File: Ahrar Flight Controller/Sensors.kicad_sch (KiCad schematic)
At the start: 38 parts, among them U3 MS5611-01BA, U5 BMP581

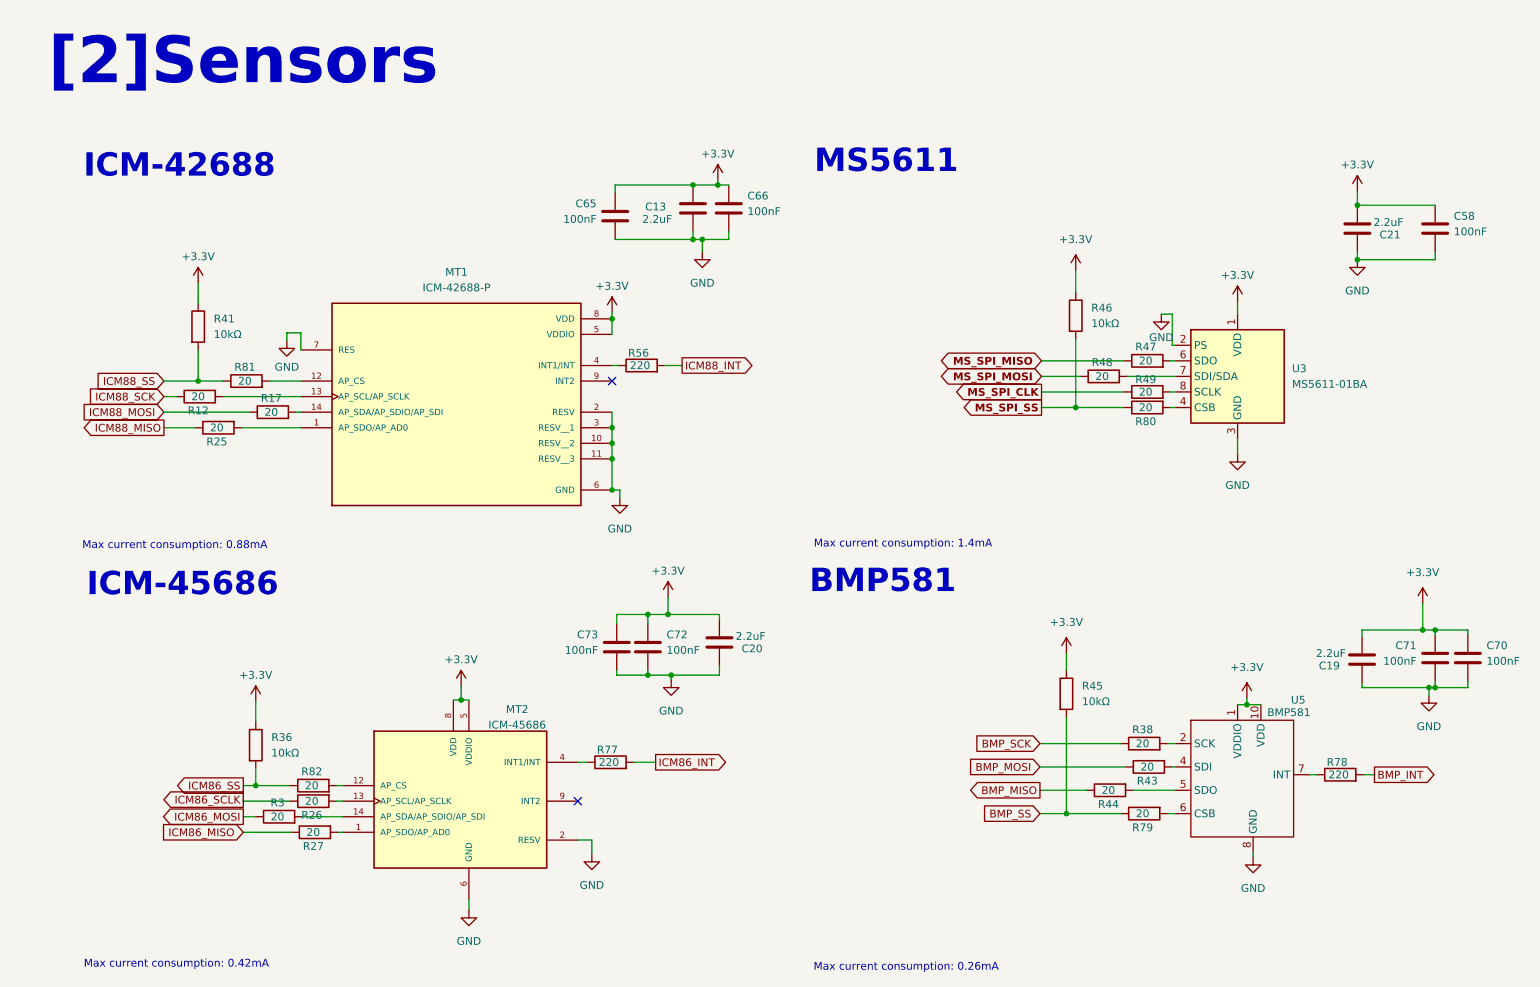
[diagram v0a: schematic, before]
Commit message: .
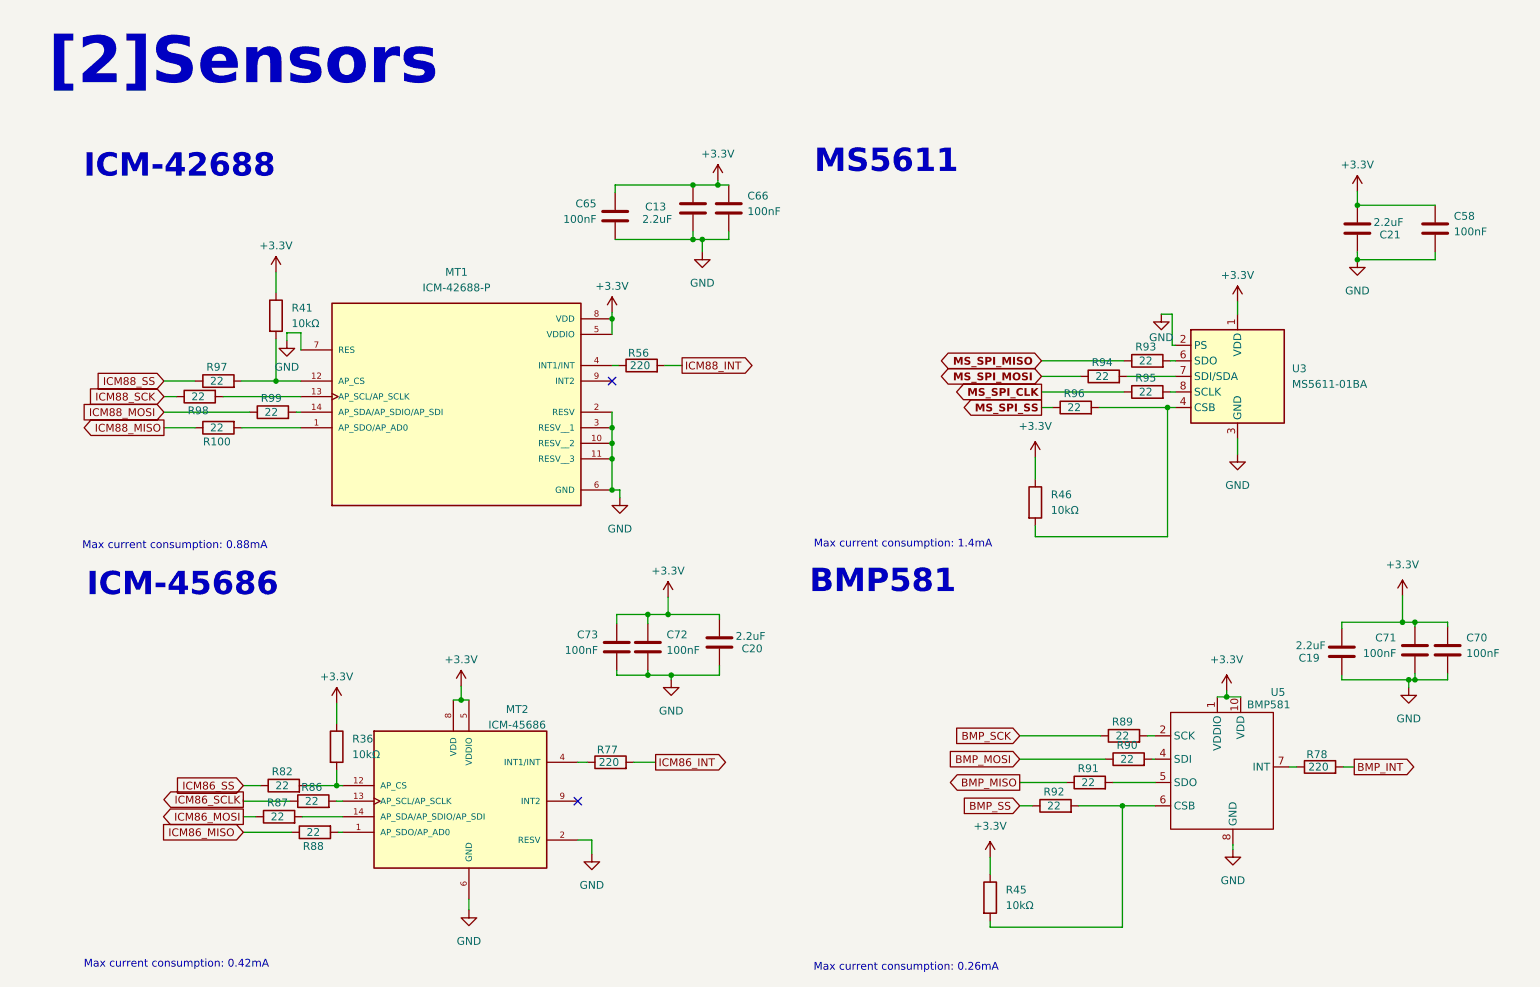
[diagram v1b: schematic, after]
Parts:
- removed R12, R17, R25, R26, R27, R3, R38, R43, R44, R47, R48, R49, R79, R80, R81: 20, Resistor_SMD:R_0402_1005Metric, symbol Device:R
- added R100, R86, R87, R88, R89, R90, R91, R92, R93, R94, R95, R96, R97, R98, R99: 22, Resistor_SMD:R_0402_1005Metric, symbol Device:R
- R82: value 20 -> 22; Distributer Link https://www.ozdisan.com/p/smt-smd-ve-cip-direncler-194/pana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 -> https://www.ozdisan.com/p/smt-smd-ve-cip-direncler-194/roya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; Part Number ERJ2GEJ200X -> CQ02WGF220JTCE
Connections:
- net BMP_MISO: now also R91.1
- net BMP_MOSI: now also R90.1
- net BMP_SCK: now also R89.1
- net BMP_SS: now also R92.1; no longer R45.2
- net ICM86_MISO: now also R88.1
- net ICM86_MOSI: now also R87.1
- net ICM86_SCLK: now also R86.1
- net ICM86_SS: no longer R36.2
- net ICM88_MISO: now also R100.1
- net ICM88_MOSI: now also R99.1
- net ICM88_SCK: now also R98.1
- net ICM88_SS: now also R97.1; no longer R41.2
- net MS_SPI_CLK: now also R95.1
- net MS_SPI_MISO: now also R93.1
- net MS_SPI_MOSI: now also R94.1
- net MS_SPI_SS: now also R96.1; no longer R46.2
- net at U5.4 (SDI): now also R90.2
- net at MT2.13 (AP_SCL/AP_SCLK): now also R86.2
- net at MT2.1 (AP_SDO/AP_AD0): now also R88.2
- net at MT2.12 (AP_CS), R82.2: now also R36.2
- net at MT2.14 (AP_SDA/AP_SDIO/AP_SDI): now also R87.2
- net at U5.2 (SCK): now also R89.2
- net at U3.7 (SDI/SDA): now also R94.2
- net at MT1.1 (AP_SDO/AP_AD0): now also R100.2
- net at U5.5 (SDO): now also R91.2
- net at MT1.14 (AP_SDA/AP_SDIO/AP_SDI): now also R99.2
- net at U5.6 (CSB): now also R45.2, R92.2
- net at MT1.12 (AP_CS): now also R41.2, R97.2
- net at MT1.13 (AP_SCL/AP_SCLK): now also R98.2
- net at U3.6 (SDO): now also R93.2
- net at U3.4 (CSB), U3.5 (CSB): now also R46.2, R96.2
- net at U3.8 (SCLK): now also R95.2
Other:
- moved on the sheet: C19, C70, C71, R36, R41, R45, R46, R78, R82, U5

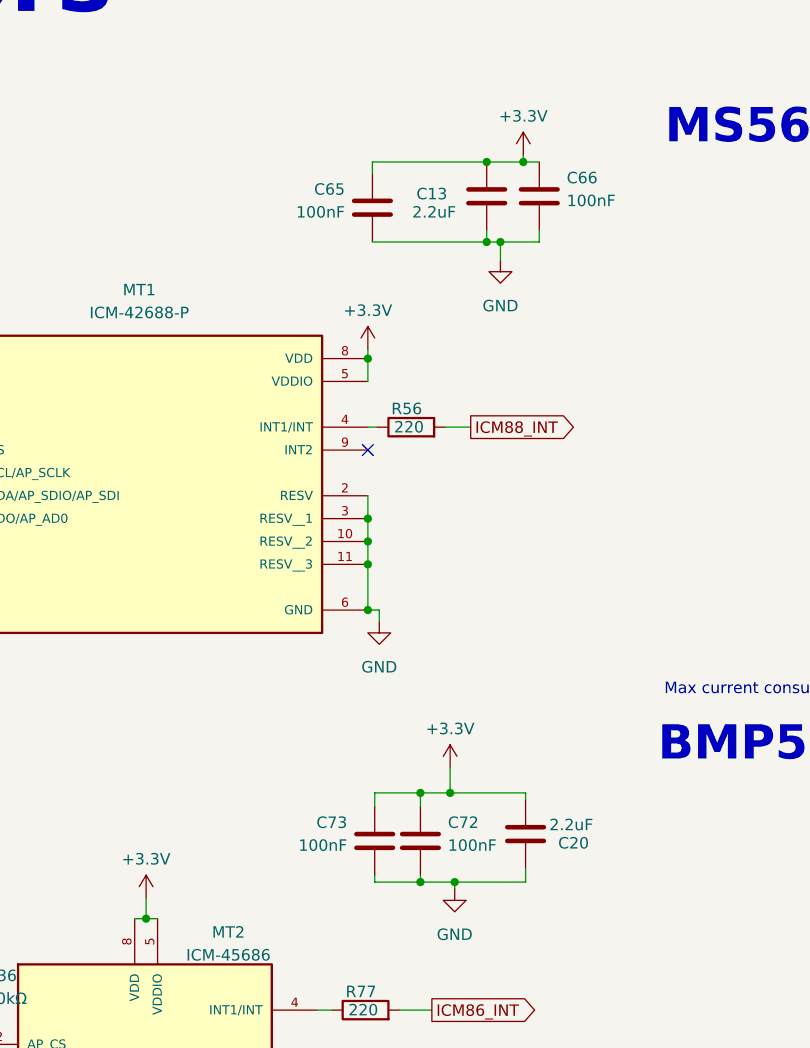
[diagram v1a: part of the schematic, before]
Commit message: .
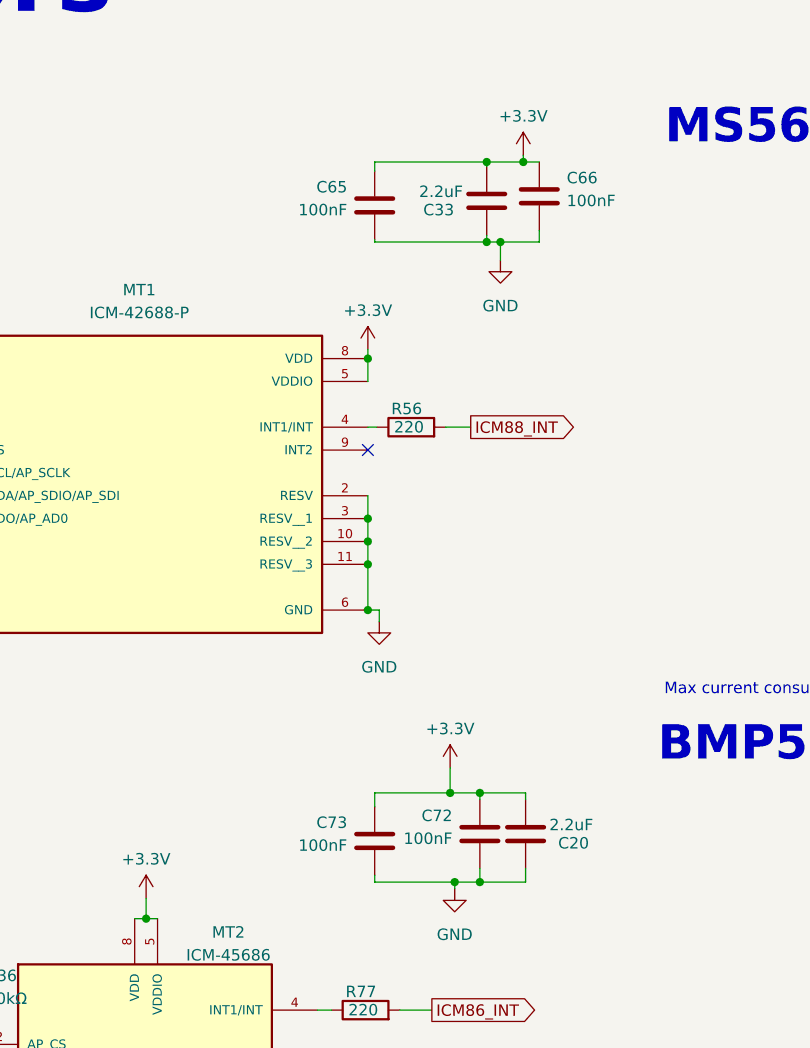
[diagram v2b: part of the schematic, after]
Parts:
- removed C13: 2.2uF, Capacitor_SMD:C_0402_1005Metric, symbol Device:C
- added C33: 2.2uF, Capacitor_SMD:C_0603_1608Metric, symbol Device:C
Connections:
- net +3.3V: now also C33.1
- net GND: now also C33.2
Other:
- moved on the sheet: C72
